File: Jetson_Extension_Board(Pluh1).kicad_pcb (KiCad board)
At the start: 2 copper layers, 25 parts, among them J1 I2C_2 DEBUG, J10 TBP03R2-350-03BE, J11 ST DEBUG, J2 TBP03R2-350-03BE, J3 TBP03R2-350-03BE, J4 TBP03R2-350-03BE, J5 TBP03R2-350-03BE, J6 40_Pin_Jetson_Connector, J7 TBP03R2-350-03BE, J8 TBP03R2-350-03BE, J9 TBP03R2-350-03BE, SW1 SW_Push_DPDT, U1 BNO055, U2 74LV14, U4 ADS1115IDGS

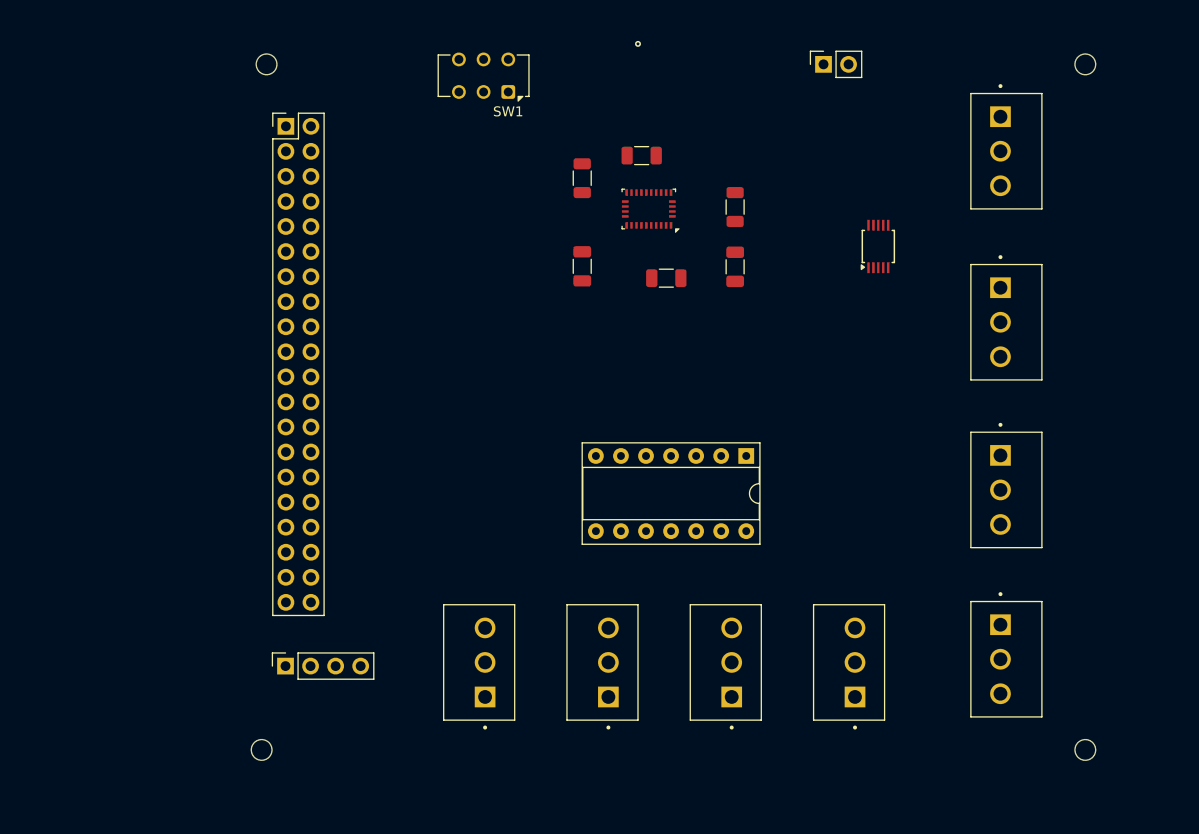
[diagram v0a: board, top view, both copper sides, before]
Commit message: Freerouted attempt
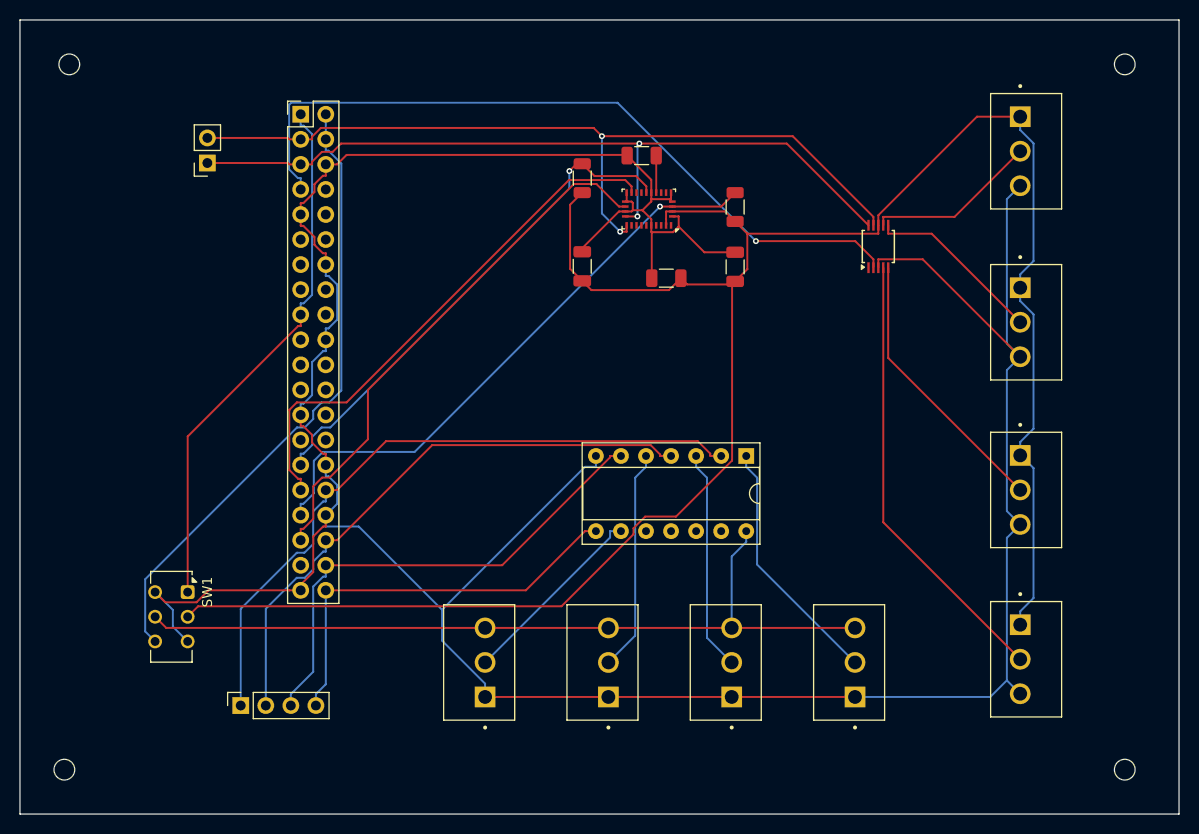
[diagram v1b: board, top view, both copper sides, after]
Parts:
- moved J1 63.3 mm to (88.5, 83.0), turned to 180 degrees
- moved SW1 60.2 mm to (86.5, 126.5), turned to -90 degrees
- moved H2 20.1 mm to (74.0, 144.5)
- moved H1 20.0 mm to (74.5, 73.0)
- moved J11 6.05 mm to (91.9, 138.0)
- moved H4 4.47 mm to (181.5, 144.5)
- moved H3 4.00 mm to (181.5, 73.0)
- moved J10 2.00 mm to (170.9, 78.3)
- moved J7 2.00 mm to (170.9, 129.8)
- moved J8 2.00 mm to (170.9, 112.6)
- moved J9 2.00 mm to (170.9, 95.6)
- moved J6 1.93 mm to (98.0, 78.1)
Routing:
- net GND: track 0.00 -> 322.5 mm
- net /ADC/3.3V: track 0.00 -> 211.2 mm
- net /I2C_2_SDA: track 0.00 -> 84.5 mm, vias 0 -> 2
- net /SchmittTrigger(74LV14)/5V: track 0.00 -> 81.8 mm
- net /I2C_2_SCL: track 0.00 -> 80.2 mm, vias 0 -> 2
- net ADC ALERT: track 0.00 -> 76.0 mm, vias 0 -> 1
- net ST 1: track 0.00 -> 68.9 mm
- net 5V: track 0.00 -> 63.8 mm
- net IMU nBOOT: track 0.00 -> 60.2 mm, vias 0 -> 1
- net ST 2: track 0.00 -> 59.4 mm
- net 3.3V: track 0.00 -> 54.6 mm
- net COM 3: track 0.00 -> 54.3 mm
- net IMU INT: track 0.00 -> 54.0 mm
- net IMU nRESET: track 0.00 -> 51.5 mm, vias 0 -> 1
- net ST 3: track 0.00 -> 50.4 mm
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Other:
- board outline added: 117.5 x 80.5 mm
